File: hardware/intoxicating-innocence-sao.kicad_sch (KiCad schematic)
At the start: 23 parts, among them J1 SAO, J2 QWIIC, U1 CH32V003F4P6

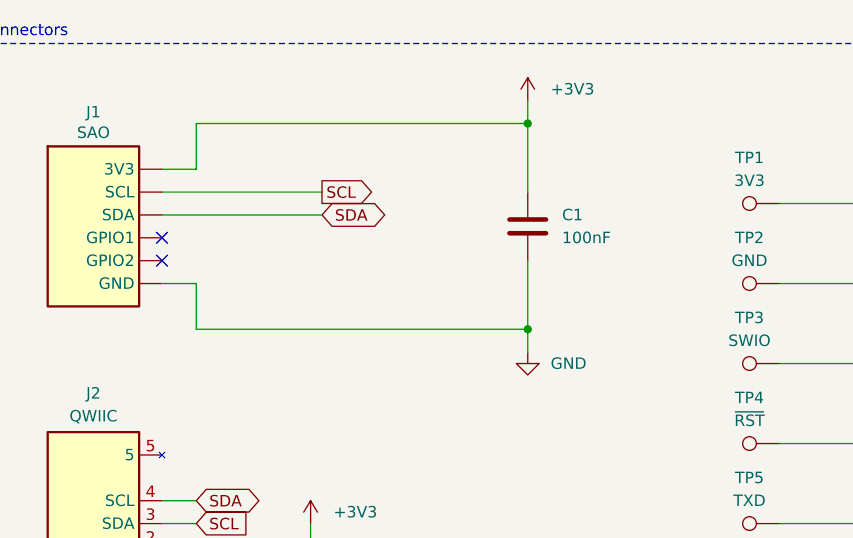
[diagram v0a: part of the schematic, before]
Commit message: Add bulk capacitor
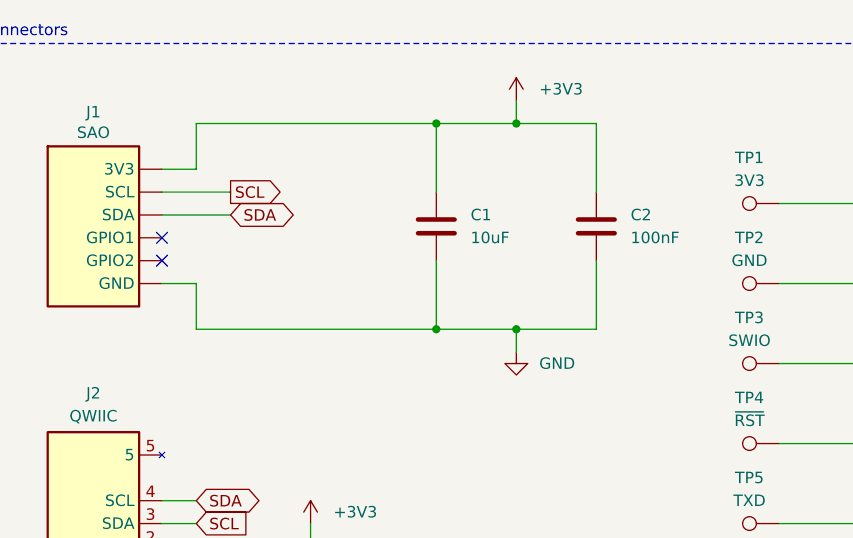
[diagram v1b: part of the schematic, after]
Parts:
- added C1: 10uF, Capacitor_SMD:C_0603_1608Metric_Pad1.08x0.95mm_HandSolder, symbol Device:C
- renumbered C1 to C2
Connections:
- net +3V3: now also C1.1
- net GND: now also C1.2
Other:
- moved on the sheet: C2
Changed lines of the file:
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@@
 	)
 	(junction
+		(at 72.39 53.34)
+		(diameter 0)
+		(color 0 0 0 0)
+	)
+	(junction
 		(at 200.66 43.18)
 		(diameter 0)
@@
 	)
 	(junction
-		(at 82.55 30.48)
+		(at 81.28 30.48)
+		(diameter 0)
+		(color 0 0 0 0)
+	)
+	(junction
+		(at 72.39 30.48)
 		(diameter 0)
 		(color 0 0 0 0)
 	)
 	(junction
-		(at 82.55 53.34)
+		(at 81.28 53.34)
 		(diameter 0)
 		(color 0 0 0 0)
@@
 	(wire
 		(pts
+			(xy 72.39 30.48) (xy 72.39 38.1)
+		)
+		(stroke
+			(width 0)
+			(type default)
+		)
+	)
+	(wire
+		(pts
 			(xy 110.49 57.15) (xy 120.65 57.15)
 		)
@@
 	(wire
 		(pts
+			(xy 72.39 30.48) (xy 90.17 30.48)
+		)
+		(stroke
+			(width 0)
+			(type default)
+		)
+	)
+	(wire
+		(pts
 			(xy 45.72 48.26) (xy 45.72 53.34)
 		)
@@
 	(wire
 		(pts
-			(xy 82.55 53.34) (xy 82.55 55.88)
+			(xy 81.28 53.34) (xy 81.28 55.88)
 		)
 		(stroke
@@
 	(wire
 		(pts
-			(xy 82.55 30.48) (xy 82.55 38.1)
+			(xy 90.17 30.48) (xy 90.17 38.1)
 		)
 		(stroke
@@
 	(wire
 		(pts
-			(xy 41.91 40.64) (xy 59.69 40.64)
+			(xy 41.91 40.64) (xy 49.53 40.64)
+		)
+		(stroke
+			(width 0)
+			(type default)
+		)
+	)
+	(wire
+		(pts
+			(xy 41.91 38.1) (xy 49.53 38.1)
 		)
 		(stroke
@@
 	(wire
 		(pts
-			(xy 41.91 38.1) (xy 59.69 38.1)
+			(xy 72.39 53.34) (xy 90.17 53.34)
 		)
 		(stroke
@@
 	(wire
 		(pts
-			(xy 82.55 53.34) (xy 45.72 53.34)
+			(xy 72.39 45.72) (xy 72.39 53.34)
+		)
+		(stroke
+			(width 0)
+			(type default)
+		)
+	)
+	(wire
+		(pts
+			(xy 45.72 53.34) (xy 72.39 53.34)
 		)
 		(stroke
@@
 	(wire
 		(pts
-			(xy 82.55 27.94) (xy 82.55 30.48)
+			(xy 81.28 27.94) (xy 81.28 30.48)
 		)
 		(stroke
@@
 	(wire
 		(pts
-			(xy 45.72 30.48) (xy 82.55 30.48)
+			(xy 45.72 30.48) (xy 72.39 30.48)
 		)
 		(stroke
@@
 	(wire
 		(pts
-			(xy 82.55 45.72) (xy 82.55 53.34)
+			(xy 90.17 45.72) (xy 90.17 53.34)
 		)
 		(stroke
@@
 	(global_label "SDA"
 		(shape bidirectional)
-		(at 59.69 40.64 0)
+		(at 49.53 40.64 0)
 		(fields_autoplaced yes)
 		(effects
@@
 		)
 		(property "Intersheetrefs" "${INTERSHEET_REFS}"
-			(at 67.3546 40.64 0)
+			(at 57.1946 40.64 0)
 			(hide yes)
 			(show_name no)
@@
 	(global_label "SCL"
 		(shape output)
-		(at 59.69 38.1 0)
+		(at 49.53 38.1 0)
 		(fields_autoplaced yes)
 		(effects
@@
 		)
 		(property "Intersheetrefs" "${INTERSHEET_REFS}"
-			(at 66.1828 38.1 0)
+			(at 56.0228 38.1 0)
 			(hide yes)
 			(show_name no)
@@
 	)
 	(symbol
+		(lib_id "Device:C")
+		(at 72.39 41.91 0)
+		(unit 1)
+		(body_style 1)
+		(exclude_from_sim no)
+		(in_bom yes)
+		(on_board yes)
+		(in_pos_files yes)
+		(dnp no)
+		(fields_autoplaced yes)
+		(property "Reference" "C1"
+			(at 76.2 40.6399 0)
+			(show_name no)
+			(do_not_autoplace no)
+			(effects
+				(font
+					(size 1.27 1.27)
+				)
+				(justify left)
+			)
+		)
+		(property "Value" "10uF"
+			(at 76.2 43.1799 0)
+			(show_name no)
+			(do_not_autoplace no)
+			(effects
+				(font
+					(size 1.27 1.27)
+				)
+				(justify left)
+			)
+		)
+		(property "Footprint" "Capacitor_SMD:C_0603_1608Metric_Pad1.08x0.95mm_HandSolder"
+			(at 73.3552 45.72 0)
+			(hide yes)
+			(show_name no)
+			(do_not_autoplace no)
+			(effects
+				(font
+					(size 1.27 1.27)
+				)
+			)
+		)
+		(property "Datasheet" ""
+			(at 72.39 41.91 0)
+			(hide yes)
+			(show_name no)
+			(do_not_autoplace no)
+			(effects
+				(font
+					(size 1.27 1.27)
+				)
+			)
+		)
+		(property "Description" "Unpolarized capacitor"
+			(at 72.39 41.91 0)
+			(hide yes)
+			(show_name no)
+			(do_not_autoplace no)
+			(effects
+				(font
+					(size 1.27 1.27)
+				)
+			)
+		)
+		(property "LCSC Part #" "C109455"
+			(at 72.39 41.91 0)
+			(hide yes)
+			(show_name no)
+			(do_not_autoplace no)
+			(effects
+				(font
+					(size 1.27 1.27)
+				)
+			)
+		)
+		(pin "1"
+		)
+		(pin "2"
+		)
+		(instances
+			(project "intoxicating-innocence-sao"
+				(path "/559a265e-8809-44d3-9227-9bc29ae1c837"
+					(reference "C1")
+					(unit 1)
+				)
+			)
+		)
+	)
+	(symbol
 		(lib_id "Device:R")
 		(at 250.19 35.56 90)
@@
 	(symbol
 		(lib_id "Device:C")
-		(at 82.55 41.91 0)
+		(at 90.17 41.91 0)
 		(unit 1)
 		(body_style 1)
@@
 		(dnp no)
 		(fields_autoplaced yes)
-		(property "Reference" "C1"
-			(at 86.36 40.6399 0)
+		(property "Reference" "C2"
+			(at 93.98 40.6399 0)
 			(show_name no)
 			(do_not_autoplace no)
@@
 		)
 		(property "Value" "100nF"
-			(at 86.36 43.1799 0)
+			(at 93.98 43.1799 0)
 			(show_name no)
 			(do_not_autoplace no)
@@
 		)
 		(property "Footprint" "Capacitor_SMD:C_0603_1608Metric_Pad1.08x0.95mm_HandSolder"
-			(at 83.5152 45.72 0)
+			(at 91.1352 45.72 0)
 			(hide yes)
 			(show_name no)
@@
 		)
 		(property "Datasheet" ""
-			(at 82.55 41.91 0)
+			(at 90.17 41.91 0)
 			(hide yes)
 			(show_name no)
@@
 		)
 		(property "Description" "Unpolarized capacitor"
-			(at 82.55 41.91 0)
+			(at 90.17 41.91 0)
 			(hide yes)
 			(show_name no)
@@
 		)
 		(property "LCSC Part #" "C14663"
-			(at 82.55 41.91 0)
+			(at 90.17 41.91 0)
 			(hide yes)
 			(show_name no)
@@
 			(project "intoxicating-innocence-sao"
 				(path "/559a265e-8809-44d3-9227-9bc29ae1c837"
-					(reference "C1")
+					(reference "C2")
 					(unit 1)
 				)
@@
 	(symbol
 		(lib_id "power:+3V3")
-		(at 82.55 27.94 0)
+		(at 81.28 27.94 0)
 		(unit 1)
 		(body_style 1)
@@
 		(fields_autoplaced yes)
 		(property "Reference" "#PWR03"
-			(at 82.55 31.75 0)
+			(at 81.28 31.75 0)
 			(hide yes)
 			(show_name no)
@@
 		)
 		(property "Value" "+3V3"
-			(at 85.09 26.6699 0)
+			(at 83.82 26.6699 0)
 			(show_name no)
 			(do_not_autoplace no)
@@
 		)
 		(property "Footprint" ""
-			(at 82.55 27.94 0)
+			(at 81.28 27.94 0)
 			(hide yes)
 			(show_name no)
@@
 		)
 		(property "Datasheet" ""
-			(at 82.55 27.94 0)
+			(at 81.28 27.94 0)
 			(hide yes)
 			(show_name no)
@@
 		)
 		(property "Description" "Power symbol creates a global label with name \"+3V3\""
-			(at 82.55 27.94 0)
+			(at 81.28 27.94 0)
 			(hide yes)
 			(show_name no)
@@
 	(symbol
 		(lib_id "power:GND")
-		(at 82.55 55.88 0)
+		(at 81.28 55.88 0)
 		(unit 1)
 		(body_style 1)
@@
 		(fields_autoplaced yes)
 		(property "Reference" "#PWR04"
-			(at 82.55 62.23 0)
+			(at 81.28 62.23 0)
 			(hide yes)
 			(show_name no)
@@
 		)
 		(property "Value" "GND"
-			(at 85.09 57.1499 0)
+			(at 83.82 57.1499 0)
 			(show_name no)
 			(do_not_autoplace no)
@@
 		)
 		(property "Footprint" ""
-			(at 82.55 55.88 0)
+			(at 81.28 55.88 0)
 			(hide yes)
 			(show_name no)
@@
 		)
 		(property "Datasheet" ""
-			(at 82.55 55.88 0)
+			(at 81.28 55.88 0)
 			(hide yes)
 			(show_name no)
@@
 		)
 		(property "Description" "Power symbol creates a global label with name \"GND\" , ground"
-			(at 82.55 55.88 0)
+			(at 81.28 55.88 0)
 			(hide yes)
 			(show_name no)
